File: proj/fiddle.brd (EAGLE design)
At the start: 71.3 x 15.2 mm, 24 parts, among them J1 DM3D-SFDM, SW6 TACTSW_2MICRO3X6, SW7 TACTSW_2MICRO3X6, U1 MCP23008QFN, U2 WRL-13678WRL-13678-QUIET, U4 3.3V 600mA

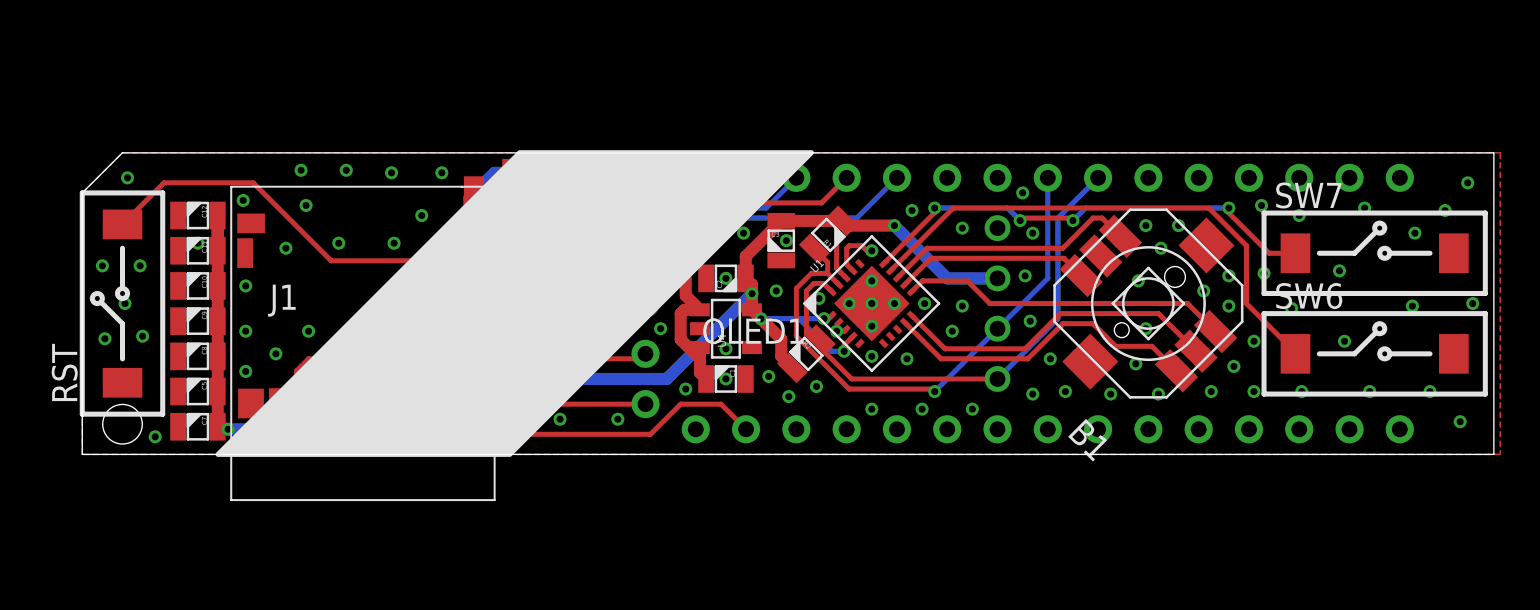
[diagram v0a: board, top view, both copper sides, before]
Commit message: tootoot
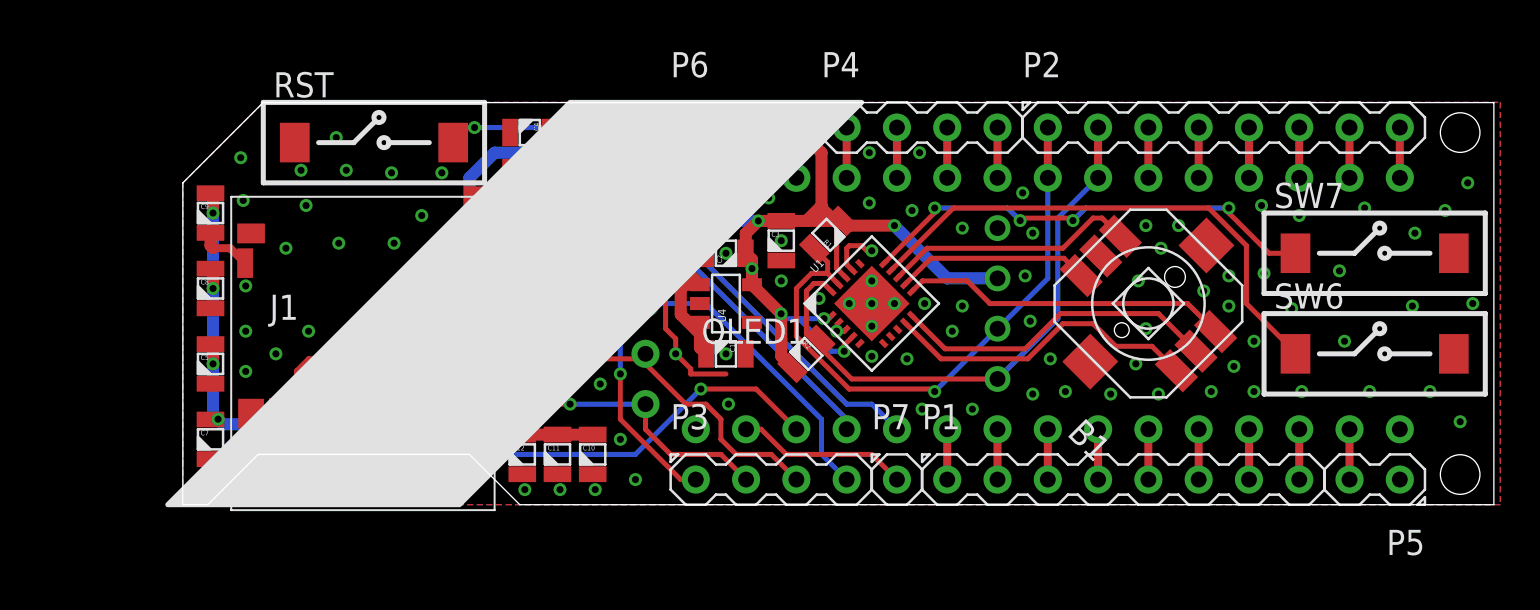
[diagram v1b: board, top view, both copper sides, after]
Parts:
- added P1, P2: PIN_8, dooba:PIN_8
- added P3, P4: PIN_4, dooba:PIN_4
- added P5: PIN_2, dooba:PIN_2
- added P6: PIN_3, dooba:PIN_3
- added P7: PIN_1, dooba:PIN_1
- moved C10 21.7 mm to (41.8, 33.0), turned to 270 degrees
- moved C11 20.9 mm to (40.0, 33.0), turned to 270 degrees
- moved C12 20.3 mm to (38.2, 33.0), turned to 270 degrees
- moved RST 15.1 mm to (30.7, 48.8), turned to 0 degrees
- moved C9 5.50 mm to (22.5, 45.2), turned to 270 degrees
- moved C8 3.49 mm to (22.5, 41.4), turned to 270 degrees
- moved C6 3.30 mm to (38.6, 47.2), turned to 180 degrees
- moved C4 2.03 mm to (38.6, 49.3)
- moved C5 1.53 mm to (22.5, 37.6), turned to 270 degrees
- moved C1 1.27 mm to (48.5, 38.1)
- moved C2 1.27 mm to (48.5, 43.2)
- moved U4 1.27 mm to (48.5, 40.6)
- moved C7 0.90 mm to (22.5, 33.8), turned to 270 degrees
- moved J1 0.51 mm to (30.2, 36.3)
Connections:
- removed net 5.5V: C1.2, N1.16, U4.1, U4.3
- new net N$10: N1.29, P2.7
- new net N$11: N1.28, P2.6
- new net N$12: N1.27, P2.5
- new net N$13: N1.26, P2.4
- new net N$14: N1.25, P2.3
- new net N$15: N1.3, P1.8
- new net N$16: N1.4, P1.7
- new net N$17: N1.5, P1.6
- new net N$18: N1.6, P1.5
- new net N$19: N1.7, P1.4
- new net N$20: N1.8, P1.3
- new net N$21: N1.9, P1.2
- new net N$22: N1.10, P1.1
- new net N$23: N1.22, P4.4
- new net N$24: N1.21, P4.3
- new net N$25: N1.20, P4.2
- new net N$26: N1.19, P4.1
- new net N$27: N1.14, P7.1
- new net N$9: N1.30, P2.8
- new net VIN: C1.2, N1.16, P6.2, U4.1, U4.3
- new net VUSB: N1.2, P5.2
- net 3.3V: now also P6.3
- net GND: now also P5.1, P6.1
- net I2C_SCL: now also P2.1
- net I2C_SDA: now also P2.2
- net MICROSD_CS: now also N1.13; no longer N1.14
- net N$8: now also P3.1
- net SPI_MISO: now also P3.3
- net SPI_MOSI: now also P3.2
- net SPI_SCK: now also P3.4
- net WIFI_FLASH: now also N1.11; no longer N1.20
- net WIFI_RST: now also N1.12; no longer N1.19
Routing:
- net VIN: track 0.00 -> 15.7 mm
- net SPI_SCK: track 18.6 -> 34.0 mm
- net 3.3V: track 99.9 -> 114.6 mm, vias 9 -> 13
- net 5.5V: track 12.6 -> 0.00 mm
- net SPI_MISO: track 19.7 -> 31.4 mm
- net GND: track 3.38 -> 13.3 mm, vias 110 -> 107
- net N$27: track 0.00 -> 8.67 mm
- net SPI_MOSI: track 15.4 -> 23.3 mm, vias 0 -> 1
- net WIFI_RST: track 17.3 -> 21.9 mm, vias 2 -> 0
- net WIFI_FLASH: track 22.2 -> 26.5 mm, vias 1 -> 0
- net MICROSD_CS: track 19.6 -> 23.4 mm, vias 0 -> 2
- net VUSB: track 0.00 -> 2.54 mm
- net N$9: track 0.00 -> 2.54 mm
- net N$26: track 0.00 -> 2.54 mm
- net N$25: track 0.00 -> 2.54 mm
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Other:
- board size 71.3 x 15.2 mm -> 66.2 x 20.3 mm
